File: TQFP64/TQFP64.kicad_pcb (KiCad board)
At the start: 2 copper layers, 81.3 x 20.3 mm, 12 parts, among them J1 Conn_01x32, J2 Conn_02x32_Counter_Clockwise, J3 Conn_02x32_Counter_Clockwise, J4 Conn_02x32_Counter_Clockwise, J5 Conn_01x32, J6 Conn_01x06

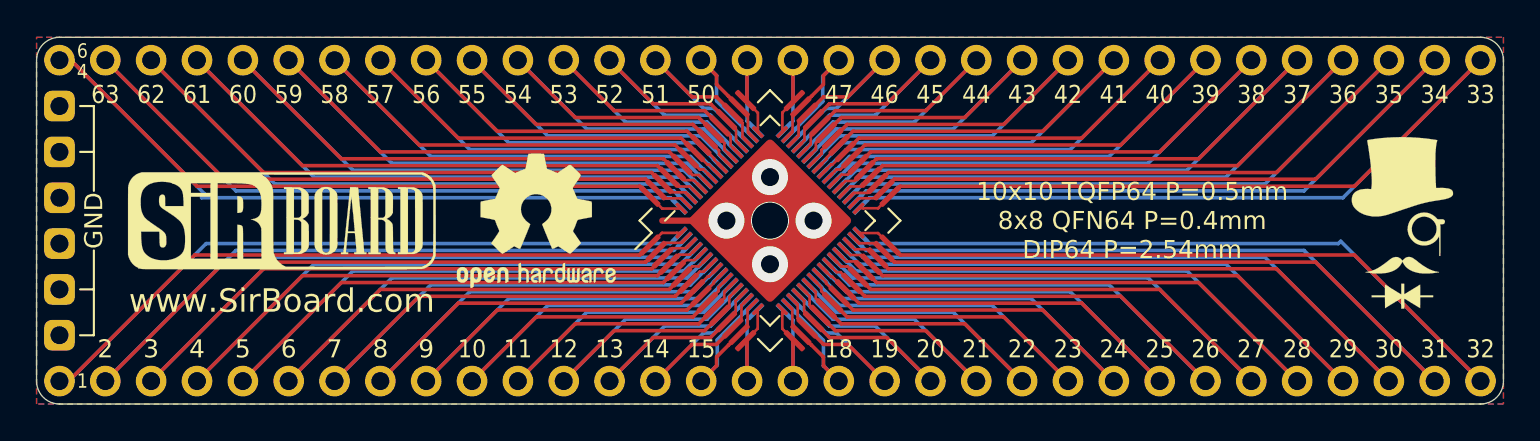
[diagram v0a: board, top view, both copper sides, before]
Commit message: apdate all footprints an run drc
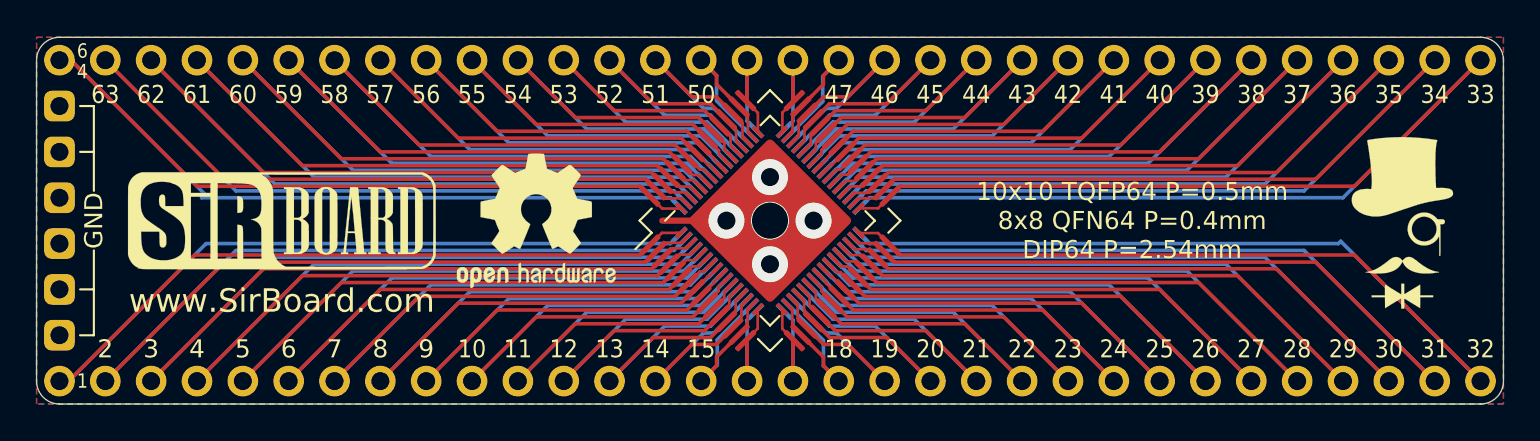
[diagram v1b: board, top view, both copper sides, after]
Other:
- net class Default removed
